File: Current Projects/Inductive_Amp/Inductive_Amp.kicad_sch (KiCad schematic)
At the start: 10 parts, among them J1 Conn_01x03, J2 Conn_01x03, U1 NA555D, U2 74LS14, U3 TLV2372

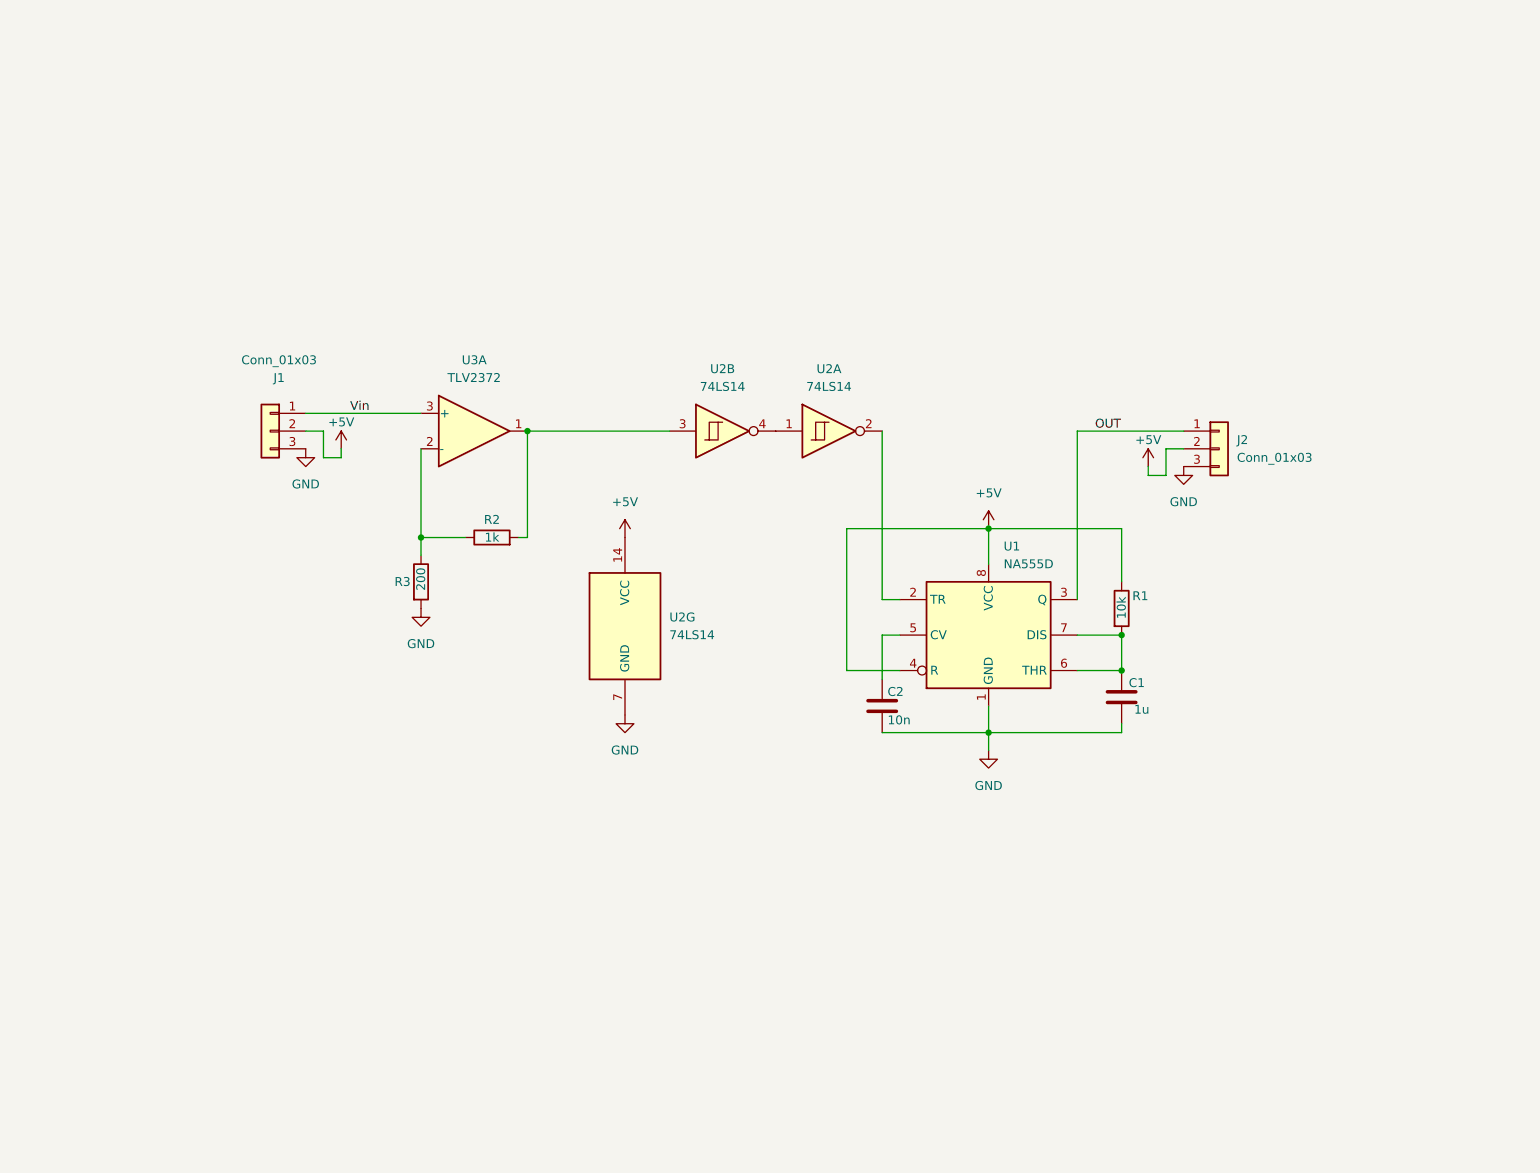
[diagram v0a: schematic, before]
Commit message: Inductive PCB!
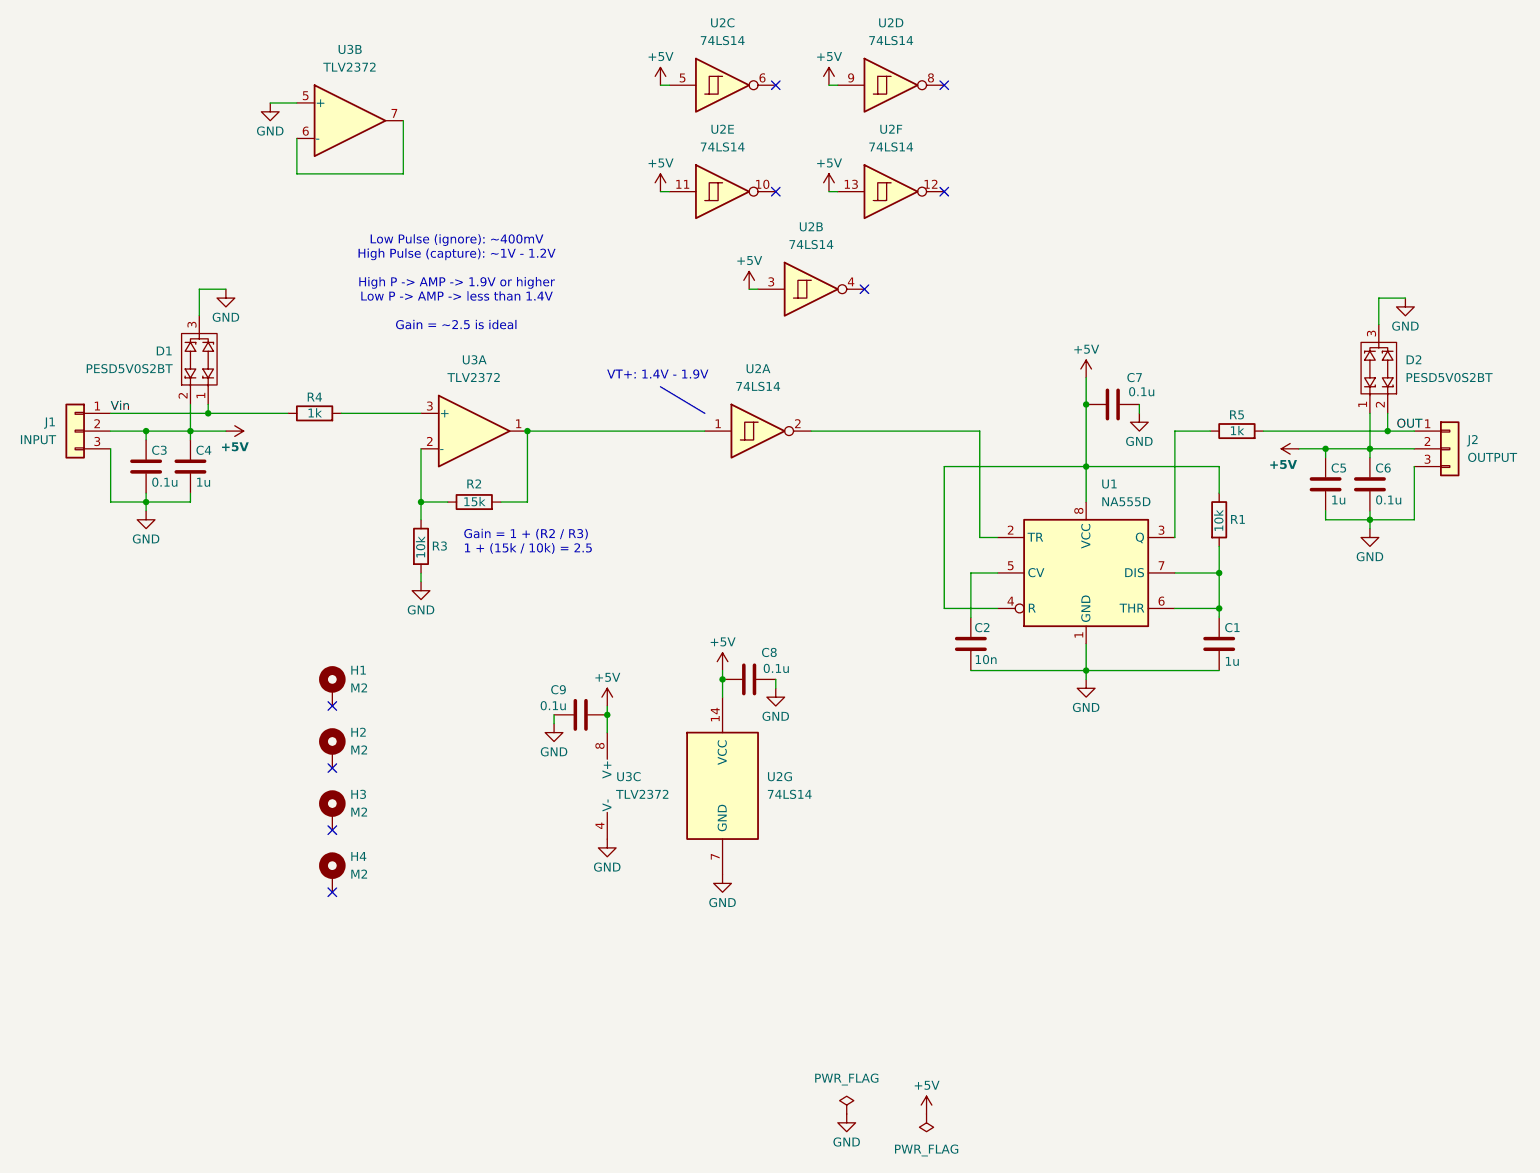
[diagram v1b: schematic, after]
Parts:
- added C3, C6, C7, C8, C9: 0.1u, Capacitor_SMD:C_0805_2012Metric, symbol Device:C
- added C4, C5: 1u, Capacitor_SMD:C_0805_2012Metric, symbol Device:C
- added D1, D2: PESD5V0S2BT, Package_TO_SOT_SMD:SOT-23-3, symbol Custom_Power_Protection:PESD5V0S2BT
- added H1, H2, H3, H4: M2, MountingHole:MountingHole_2.2mm_M2_DIN965_Pad, symbol Mechanical:MountingHole_Pad
- added R4, R5: 1k, Resistor_SMD:R_0805_2012Metric, symbol Device:R
- added unit 6 of U2
- added unit 4 of U2
- added unit 5 of U2
- added unit 3 of U2
- added unit 3 of U3
- added unit 2 of U3
- J1: value Conn_01x03 -> INPUT
- J2: value Conn_01x03 -> OUTPUT
- R2: value 1k -> 15k
- R3: value 200 -> 10k
- U2: footprint Package_SO:SOIC-14_3.9x8.7mm_P1.27mm -> (none)
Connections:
- net +5V: now also U2.3, C3.1, C4.1, C5.1, C6.1, C7.1, C8.1, C9.1, D1.2, D2.1, U2.11, U2.13, U2.5, U2.9, U3.8 (V+)
- net GND: now also C3.2, C4.2, C5.2, C6.2, C7.2, C8.2, C9.2, D1.3, D2.3, U3.4 (V-), U3.5 (+)
- net OUT: now also D2.2, R5.2; no longer U1.3 (Q)
- net Vin: now also D1.1, R4.1; no longer U3.3 (+)
- net at R2.2, U3.1: now also U2.1; no longer U2.3
- net at U2.4: no longer U2.1
- new net: R4.2, U3.3 (+)
- new net: U3.6 (-), U3.7
- new net: R5.1, U1.3 (Q)
- no-connect marks 0 -> 9
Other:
- note added: "Gain = 1 + (R2 / R3) 1 + (15k / 10k) = 2.5"
- note added: "Low Pulse (ignore): ~400mV High Pulse (capture): ~1V - 1.2V High P -> AMP -> 1.9V or higher Low P -> AMP -> less than 1.4V Gain = ~2.5 is ideal"
- note added: "VT+: 1.4V - 1.9V"
- moved on the sheet: C1, C2, J1, J2, R1, R2, R3, U1, U2A, U2G
